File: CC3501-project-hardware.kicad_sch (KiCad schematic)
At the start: 14 parts, among them J1 USB_C_Receptacle_USB2.0_16P, U1 RP2040, U3 CR2013-MI2120, U4 SY8089A1AAC, U7 HX711

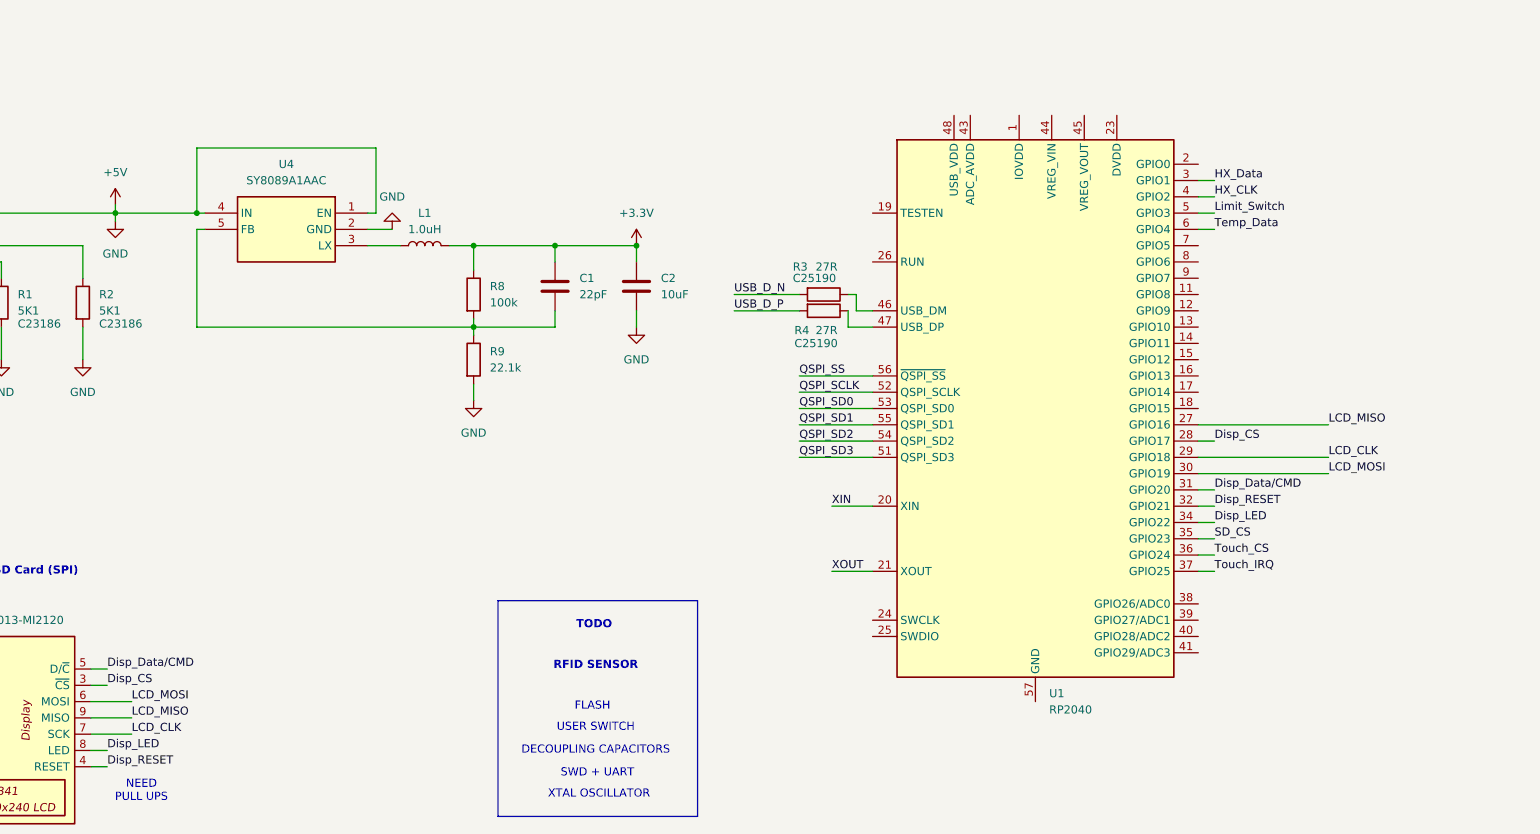
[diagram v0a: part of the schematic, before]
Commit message: finalise dc-dc step down.
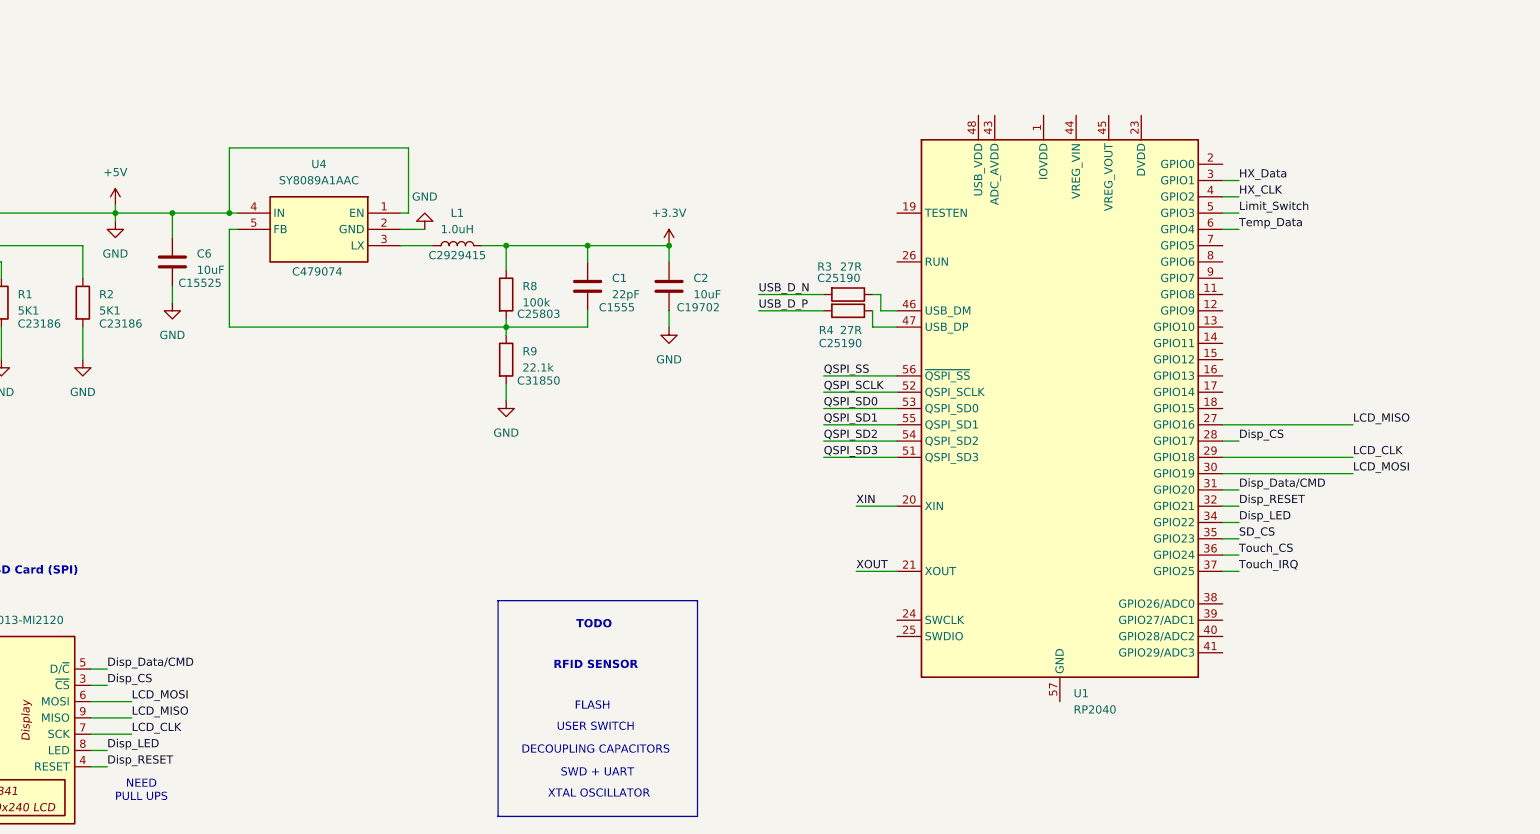
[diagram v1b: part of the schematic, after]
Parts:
- added C6: 10uF, Capacitor_SMD:C_0402_1005Metric, symbol Device:C
- C1: footprint (none) -> Capacitor_SMD:C_0402_1005Metric; LCSC PN (none) -> C1555
- C2: footprint (none) -> Capacitor_SMD:C_0603_1608Metric; LCSC PN (none) -> C19702
- L1: footprint (none) -> SamacSys_Parts:IND-SMD_L4.5-W4.0; LCSC PN (none) -> C2929415
- R8: footprint (none) -> Resistor_SMD:R_0603_1608Metric; LCSC PN (none) -> C25803
- R9: footprint (none) -> Resistor_SMD:R_0603_1608Metric; LCSC PN (none) -> C31850
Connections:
- net +5V: now also C6.1, C6.2
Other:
- moved on the sheet: C1, C2, L1, R3, R4, R8, R9, U1, U4
